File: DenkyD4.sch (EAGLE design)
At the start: 41 parts, among them J1 CON_HEADER_1X06NO_SILK, J2 CON_HEADER_1X06NO_SILK, Q1 MUN5214DW1T1G, Q2 BSS138, SW1 RESET, U1 ESP32-PICO-D4, U2 FT231XQ-R, U3 AP2112K

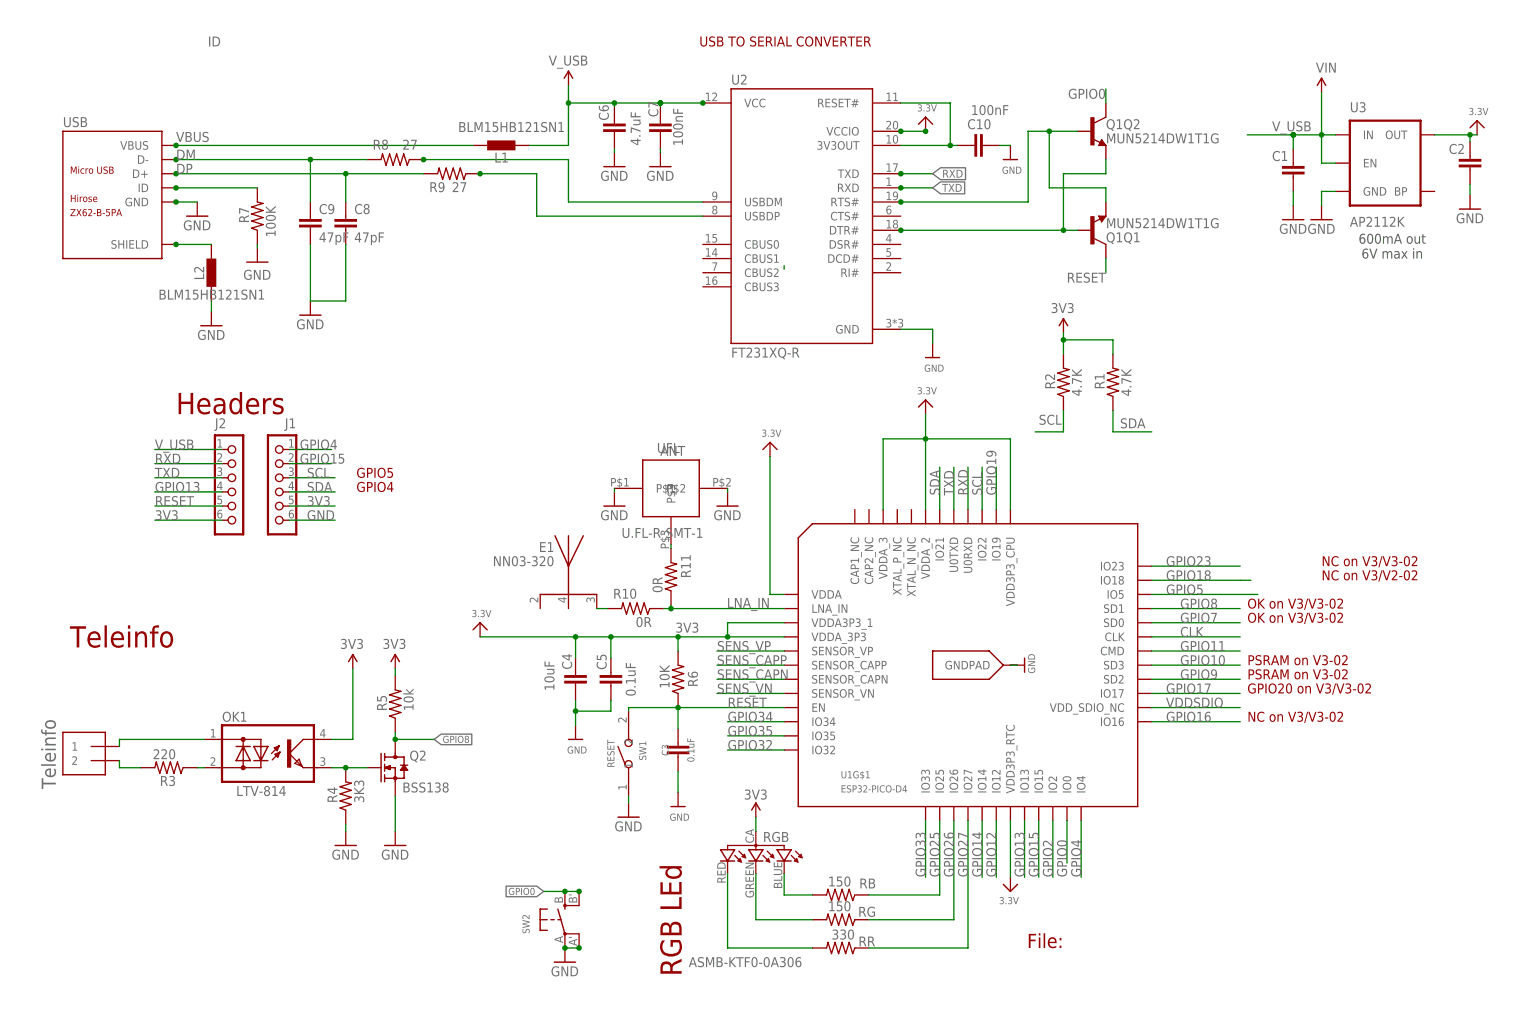
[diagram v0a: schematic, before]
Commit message: Updated to V1.2
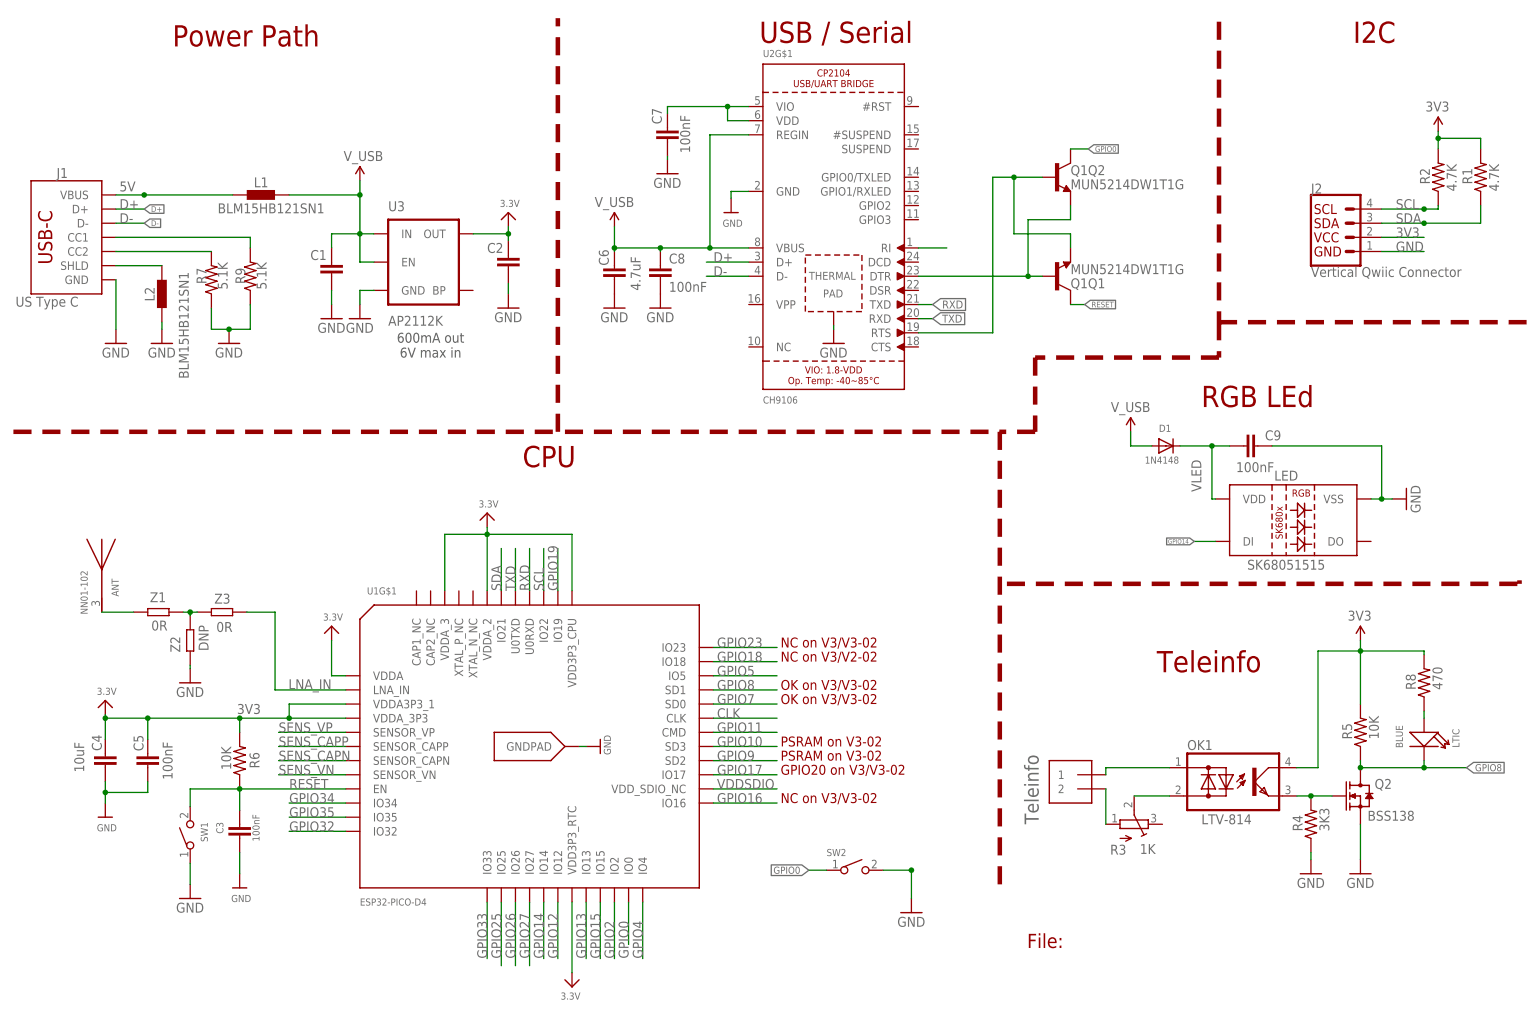
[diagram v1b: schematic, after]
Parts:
- removed C10: 100nF, _c2h:CAP0402-CAP-OK
- removed E1: NN03-320, _c2h:NN03-320
- removed R10, R11: 0R, _c2h:RESISTOR0603-RES
- removed RB, RG: 150, _c2h:RESISTOR0402-RES
- removed RGB: ASMB-KTF0-0A306, Particle:RGB-LED-CLMVB-FKARGB
- removed RR: 330, _c2h:RESISTOR0402-RES
- removed TINFO: 1X2-3.5MM, adafruit:1X2-3.5MM
- removed UFL: U.FL-R-SMT-1, Kris:U.FL-R-SMT-1
- removed USB: ZX62-B-5PA, Seeed-Connector:MICRO-USB-SMD(ZX62-B-5PA)
- added ANT: NN01-102, _c2h:NN01-102320
- added D1: 1N4148, microbuilder:DIODESOD-523
- added J3: KF2EDGR-3.81-2P, _c2h:1X2-3.5MM-3.5MM
- added LED: SK68051515, _c2h:SK68051515
- added LTIC: BLUE, OPL_Optoelectronics:SMD-LED-CLEAR-BLUE(0402)
- added Z1, Z3: 0R, _c2h:MATCHNET
- added Z2: DNP, _c2h:MATCHNET
- C3, C5: value 0.1uF -> 100nF
- C8, C9: value 47pF -> 100nF
- J1: value CON_HEADER_1X06NO_SILK -> US Type C; device _c2h:CON_HEADER_1X06NO_SILK -> SparkFun-Connectors:USB_C_4-LAYER-ISOLATED
- J2: value CON_HEADER_1X06NO_SILK -> Vertical Qwiic Connector; device _c2h:CON_HEADER_1X06NO_SILK -> _c2h:QWIIC_CONNECTOR
- Q2: device Seeed-Discrete:MOSFET-N-'' -> _c2h:SMD-MOSFET-N-CH-20V-2.1A-CJ2302(SOT-23)
- R3: value 220 -> 1K; device _c2h:RESISTOR0603-RES -> adafruit:TRIMPOTTC33X
- R5: value 10k -> 10K
- R7: value 100K -> 5.1K
- R8: value 27 -> 470; device _c2h:RESISTOR0402-RES -> LowPowerLab:RESISTOR0402-RES
- R9: value 27 -> 5.1K
- SW1: device Seeed-Switch:SMD-BUTTON(2P-3.0X2.5X1.2+0.4MM)-B3U-1000P-2P-SMD -> _c2h:SMD-BUTTON(2P-3.0X2.5X1.2+0.4MM)
- SW2: device microbuilder:SWITCH_TACT_SMT4.6X2.8 -> _c2h:SMD-BUTTON(2P-3.0X2.5X1.2+0.4MM)
- U2: value FT231XQ-R -> CH9106; device FT231XQ-R:FT231XQ-R -> microbuilder:CP2104
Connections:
- removed net ANT: R11.2, UFL.P$3
- removed net B$7: RB.2, RGB.2
- removed net DM: C9.1, R8.2, USB.D-
- removed net DP: C8.1, R9.2, USB.D+
- removed net G$6: RG.2, RGB.3
- removed net ID: R7.2, USB.ID
- removed net R$2: RGB.4, RR.2
- removed net VBUS: L1.1, USB.VBUS
- new net 5V: J1.VBUS, L1.1
- new net N$10: LTIC.+, R8.1
- new net N$11: J1.CC1, R9.2
- new net N$12: J1.CC2, R7.2
- new net N$6: U2G$1.RI
- new net N$8: C7.2, U2G$1.VDD, U2G$1.VIO
- new net VLED: C9.1, D1.C, LED.VDD
- net 3V3: now also J2.2, R8.2; no longer J1.5, J2.6, RGB.1, U2.VCCIO
- net D+: now also J1.D+, U2G$1.D+; no longer R8.1, U2.USBDM
- net D-: now also J1.D-, U2G$1.D-; no longer R9.1, U2.USBDP
- net DTR: now also U2G$1.DTR; no longer U2.DTR#
- net GND: now also J1.GND, J2.1, LED.VSS, R9.1, SW2.2, U2G$1.GND, U2G$2.TP, Z2.2; no longer C10.2, J1.6, SW2.P, SW2.P1, U2.GND, UFL.P$1, UFL.P$2, USB.GND
- net GPIO0: now also SW2.1; no longer SW2.S, SW2.S1
- net GPIO13: no longer J2.4
- net GPIO14: now also LED.DI
- net GPIO15: no longer J1.2
- net GPIO25: no longer RB.1
- net GPIO26: no longer RG.1
- net GPIO27: no longer RR.1
- net GPIO4: no longer J1.1
- net GPIO8: now also LTIC.-
- net LNA_IN: now also Z3.2; no longer R10.1, R11.1
- net N$1: now also Z1.1, Z2.1, Z3.1; no longer C10.1, U2.3V3OUT, U2.RESET#
- net N$13: now also ANT.1, Z1.2; no longer E1.FEED_BLUETOOTH, R10.2
- net N$3: now also R3.S; no longer R3.1
- net N$4: now also J3.1; no longer TINFO.1
- net N$5: now also J3.2, R3.A; no longer R3.2, TINFO.2
- net RESET: no longer J2.5
- net RTS: now also U2G$1.RTS; no longer U2.RTS#
- net RXD: now also U2G$1.TXD; no longer J2.2, U2.TXD
- net SCL: now also J2.4; no longer J1.3
- net SDA: now also J2.3; no longer J1.4
- net SHIELD: now also J1.SHLD; no longer USB.SHIELD
- net TXD: now also U2G$1.RXD; no longer J2.3, U2.RXD
- net V_USB: now also C8.1, D1.A, U2G$1.REGIN, U2G$1.VBUS; no longer C7.2, J2.1, U2.VCC
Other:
- note added: "CPU"
- note added: "I2C"
- note added: "Power Path"
- note added: "USB / Serial"
- note removed: "GPIO4"
- note removed: "GPIO5"
- note removed: "Headers"
- note removed: "USB TO SERIAL CONVERTER"
- moved on the sheet: C1, C2, C3, C4, C5, C6, C7, C8, C9, L1, L2, OK1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
